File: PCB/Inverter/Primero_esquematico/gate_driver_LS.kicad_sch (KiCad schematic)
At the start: 46 parts

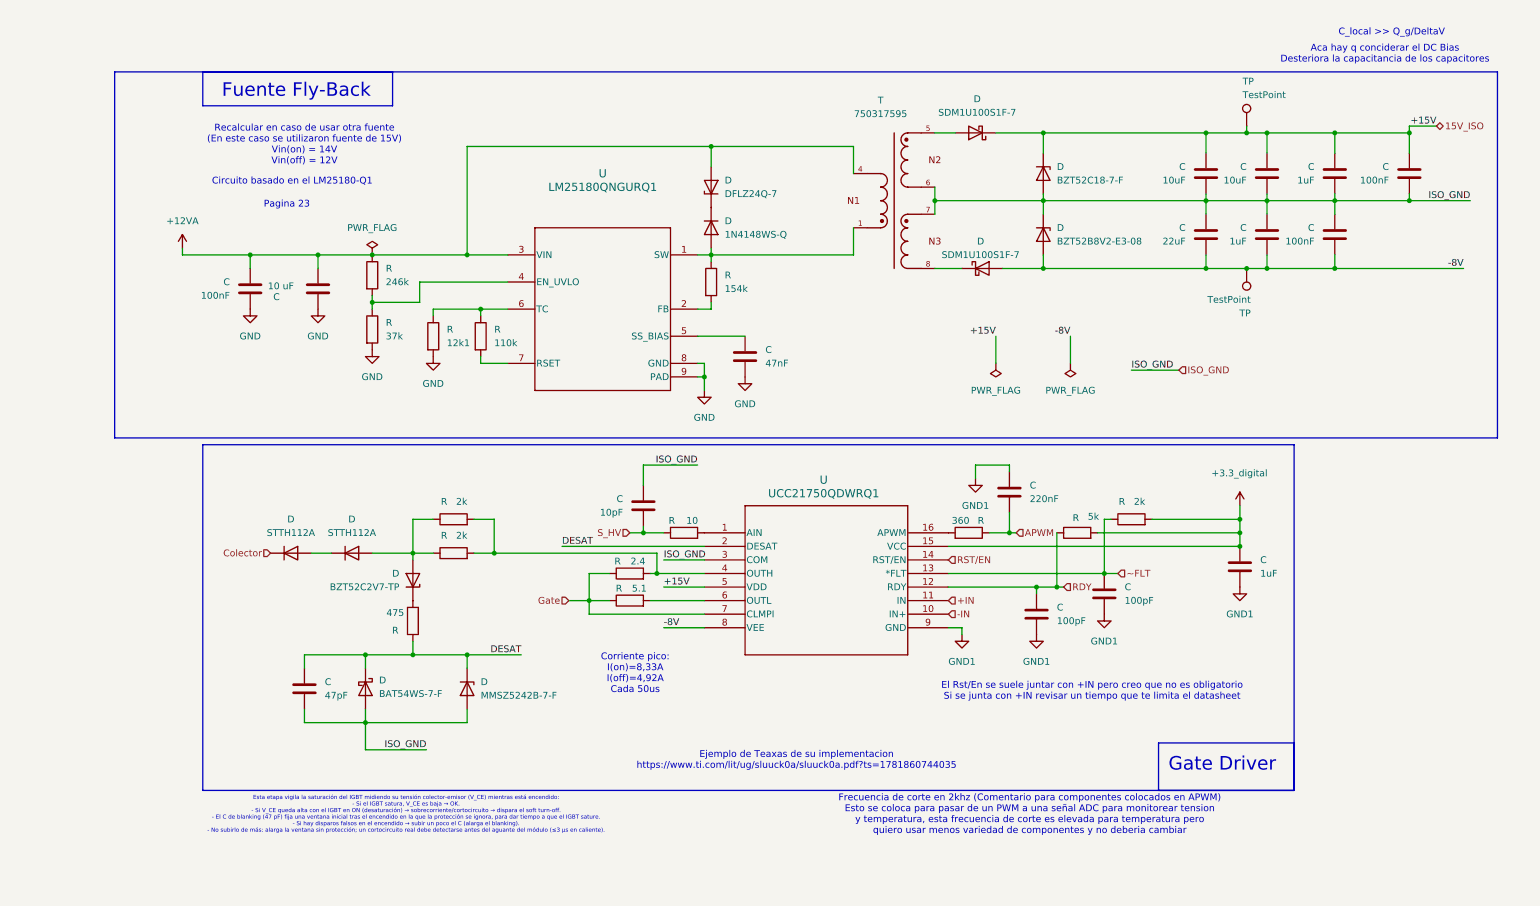
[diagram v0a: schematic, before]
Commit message: Algunos cambios
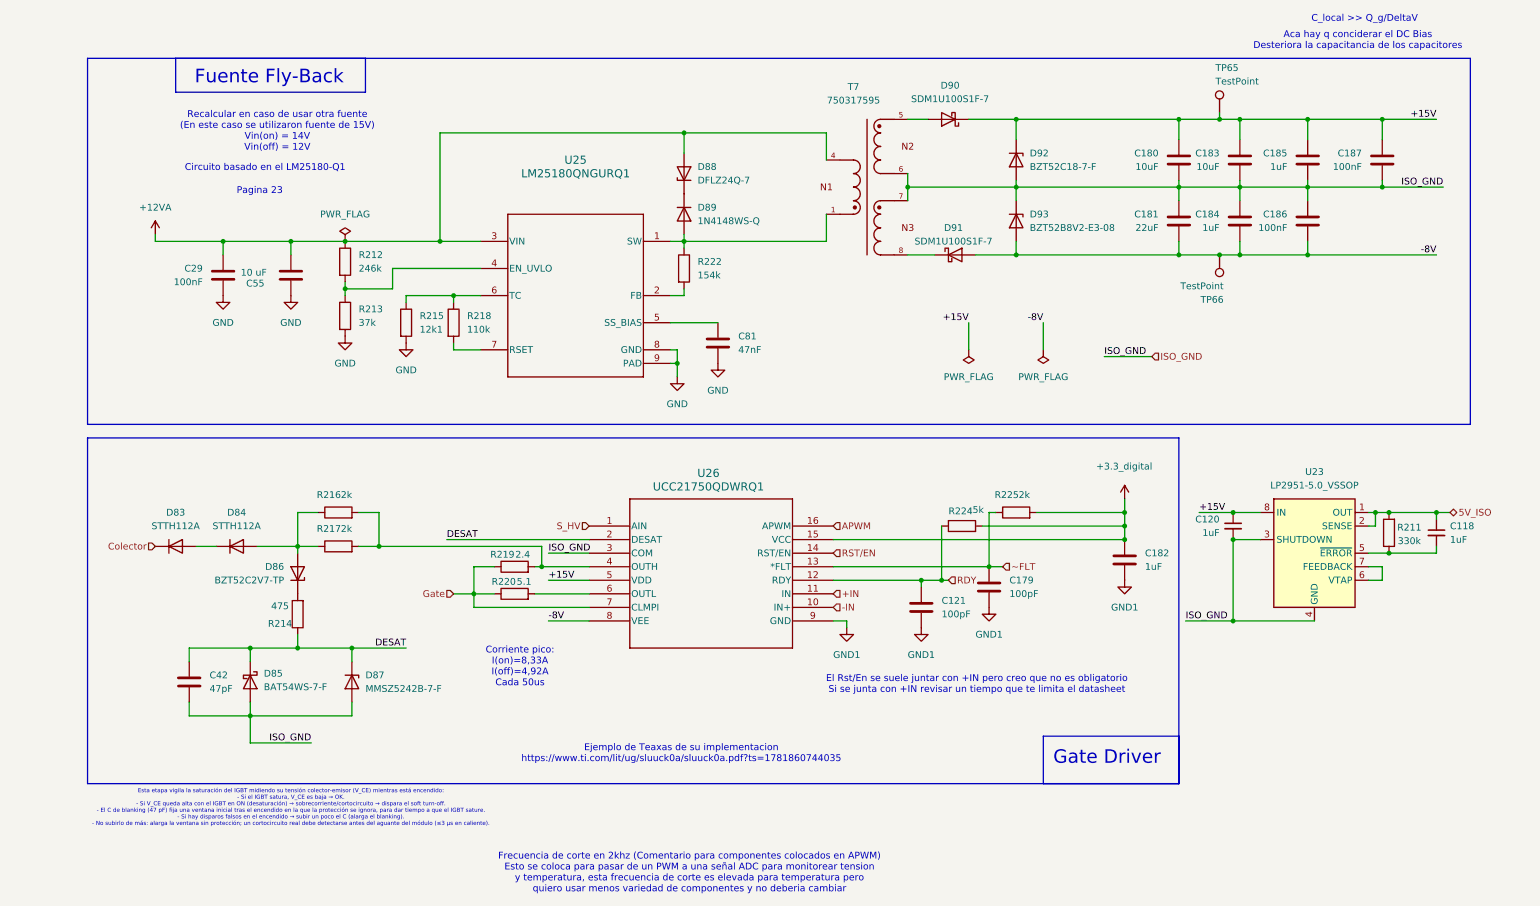
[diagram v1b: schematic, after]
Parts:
- removed C: 10 uF, Capacitor_SMD:C_1206_3216Metric, symbol Device:C
- removed C: 220nF, Capacitor_SMD:C_0402_1005Metric, symbol Device:C
- removed C: 10pF, Capacitor_SMD:C_0402_1005Metric, symbol Device:C
- removed C (x2): 1uF, Capacitor_SMD:C_0805_2012Metric, symbol Device:C
- removed C (x3): 100nF, Capacitor_SMD:C_0402_1005Metric, symbol Device:C
- removed C: 1uF, Capacitor_SMD:C_0603_1608Metric, symbol Device:C
- removed C: 47nF, Capacitor_SMD:C_0402_1005Metric_Pad0.74x0.62mm_HandSolder, symbol Device:C
- removed C: 47pF, Capacitor_SMD:C_0603_1608Metric_Pad1.08x0.95mm_HandSolder, symbol Device:C
- removed C (x2): 10uF, Capacitor_SMD:C_1210_3225Metric, symbol Device:C
- removed C: 22uF, Capacitor_SMD:C_1210_3225Metric, symbol Device:C
- removed C (x2): 100pF, Capacitor_SMD:C_0402_1005Metric, symbol Device:C
- removed D: BZT52C18-7-F, Diode_SMD:D_SOD-123, symbol Device:D_Zener
- removed D (x2): SDM1U100S1F-7, Diode_SMD:D_SOD-123F, symbol Device:D_Schottky
- removed D: MMSZ5242B-7-F, Diode_SMD:D_SOD-123, symbol Device:D_Zener
- removed D: BAT54WS-7-F, Diode_SMD:D_SOD-323_HandSoldering, symbol Device:D_Schottky
- removed D: DFLZ24Q-7, Diode_SMD:D_PowerDI-123, symbol Device:D_Zener
- removed D: 1N4148WS-Q, Diode_SMD:D_SOD-323F, symbol Device:D
- removed D (x2): STTH112A, Diode_SMD:D_SOD-323F, symbol Device:D
- removed D: BZT52B8V2-E3-08, Diode_SMD:D_SOD-123, symbol Device:D_Zener
- removed D: BZT52C2V7-TP, Diode_SMD:D_SOD-123, symbol Device:D_Zener
- removed R: 37k, Resistor_SMD:R_0402_1005Metric, symbol Device:R
- removed R: 5.1, Resistor_SMD:R_1206_3216Metric, symbol Device:R
- removed R: 110k, Resistor_SMD:R_0402_1005Metric, symbol Device:R
- removed R: 10, Resistor_SMD:R_0402_1005Metric, symbol Device:R
- removed R (x2): 2k, Resistor_SMD:R_0805_2012Metric, symbol Device:R
- removed R: 2.4, Resistor_SMD:R_1206_3216Metric, symbol Device:R
- removed R: 246k, Resistor_SMD:R_0402_1005Metric, symbol Device:R
- removed R: 360, Resistor_SMD:R_0402_1005Metric, symbol Device:R
- removed R: 154k, Resistor_SMD:R_0402_1005Metric_Pad0.72x0.64mm_HandSolder, symbol Device:R
- removed R: 475, Resistor_SMD:R_0805_2012Metric, symbol Device:R
- removed R: 12k1, Resistor_SMD:R_0402_1005Metric, symbol Device:R
- removed R: 5k, Resistor_SMD:R_0402_1005Metric, symbol Device:R
- removed R: 2k, Resistor_SMD:R_0402_1005Metric, symbol Device:R
- removed T: 750317595, Snapeda:WE-FLYTI_EP7_4436, symbol Snapeda:750317595
- removed TP (x2): TestPoint, TestPoint:TestPoint_Pad_D1.0mm, symbol Connector:TestPoint
- removed U: UCC21750QDWRQ1, Snapeda:SOIC16_DW_TEX-L, symbol Snapeda:UCC21750QDWRQ1
- removed U: LM25180QNGURQ1, Snapeda:NGU0008C, symbol Snapeda:LM25180QNGURQ1
- added C118, C120: 1uF, Capacitor_SMD:C_0603_1608Metric, symbol Device:C_Small
- added C121, C179: 100pF, Capacitor_SMD:C_0402_1005Metric, symbol Device:C
- added C180, C183: 10uF, Capacitor_SMD:C_1210_3225Metric, symbol Device:C
- added C181: 22uF, Capacitor_SMD:C_1210_3225Metric, symbol Device:C
- added C182: 1uF, Capacitor_SMD:C_0603_1608Metric, symbol Device:C
- added C184, C185: 1uF, Capacitor_SMD:C_0805_2012Metric, symbol Device:C
- added C186, C187, C29: 100nF, Capacitor_SMD:C_0402_1005Metric, symbol Device:C
- added C42: 47pF, Capacitor_SMD:C_0603_1608Metric_Pad1.08x0.95mm_HandSolder, symbol Device:C
- added C55: 10 uF, Capacitor_SMD:C_1206_3216Metric, symbol Device:C
- added C81: 47nF, Capacitor_SMD:C_0402_1005Metric_Pad0.74x0.62mm_HandSolder, symbol Device:C
- added D83, D84: STTH112A, Diode_SMD:D_SOD-323F, symbol Device:D
- added D85: BAT54WS-7-F, Diode_SMD:D_SOD-323_HandSoldering, symbol Device:D_Schottky
- added D86: BZT52C2V7-TP, Diode_SMD:D_SOD-123, symbol Device:D_Zener
- added D87: MMSZ5242B-7-F, Diode_SMD:D_SOD-123, symbol Device:D_Zener
- added D88: DFLZ24Q-7, Diode_SMD:D_PowerDI-123, symbol Device:D_Zener
- added D89: 1N4148WS-Q, Diode_SMD:D_SOD-323F, symbol Device:D
- added D90, D91: SDM1U100S1F-7, Diode_SMD:D_SOD-123F, symbol Device:D_Schottky
- added D92: BZT52C18-7-F, Diode_SMD:D_SOD-123, symbol Device:D_Zener
- added D93: BZT52B8V2-E3-08, Diode_SMD:D_SOD-123, symbol Device:D_Zener
- added R211: 330k, Resistor_SMD:R_0402_1005Metric, symbol Device:R
- added R212: 246k, Resistor_SMD:R_0402_1005Metric, symbol Device:R
- added R213: 37k, Resistor_SMD:R_0402_1005Metric, symbol Device:R
- added R214: 475, Resistor_SMD:R_0805_2012Metric, symbol Device:R
- added R215: 12k1, Resistor_SMD:R_0402_1005Metric, symbol Device:R
- added R216, R217: 2k, Resistor_SMD:R_0805_2012Metric, symbol Device:R
- added R218: 110k, Resistor_SMD:R_0402_1005Metric, symbol Device:R
- added R219: 2.4, Resistor_SMD:R_1206_3216Metric, symbol Device:R
- added R220: 5.1, Resistor_SMD:R_1206_3216Metric, symbol Device:R
- added R222: 154k, Resistor_SMD:R_0402_1005Metric_Pad0.72x0.64mm_HandSolder, symbol Device:R
- added R224: 5k, Resistor_SMD:R_0402_1005Metric, symbol Device:R
- added R225: 2k, Resistor_SMD:R_0402_1005Metric, symbol Device:R
- added T7: 750317595, Snapeda:WE-FLYTI_EP7_4436, symbol Snapeda:750317595
- added TP65, TP66: TestPoint, TestPoint:TestPoint_Pad_D1.0mm, symbol Connector:TestPoint
- added U23: LP2951-5.0_VSSOP, Package_SO:VSSOP-8_3x3mm_P0.65mm, symbol Regulator_Linear:LP2951-5.0_VSSOP
- added U25: LM25180QNGURQ1, Snapeda:NGU0008C, symbol Snapeda:LM25180QNGURQ1
- added U26: UCC21750QDWRQ1, Snapeda:SOIC16_DW_TEX-L, symbol Snapeda:UCC21750QDWRQ1
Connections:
- net +12VA: now also C29.2, C55.1, D88.2 (A), R212.1, T7.4, U25.3 (VIN)
- net +3.3_digital: now also C182.2, R224.2, R225.2, U26.15 (VCC)
- net +IN: now also U26.11 (IN)
- net -8V: now also C181.1, C184.1, C186.1, D91.2 (A), D93.2 (A), TP66.1, U26.8 (VEE)
- net -IN: now also U26.10 (IN+)
- net APWM: now also U26.16 (APWM)
- net Colector: now also D83.1 (K)
- net DESAT: now also C42.2, D85.1 (K), D87.1 (K), R214.1, U26.2 (DESAT)
- net GND: now also C29.1, C55.2, C81.1, R213.2, R215.2, U25.8 (GND), U25.9 (PAD)
- net GND1: now also C121.1, C179.1, C182.1, U26.9 (GND)
- net Gate: now also R219.1, R220.1, U26.7 (CLMPI)
- net ISO_GND: now also C120.2, C180.1, C181.2, C183.1, C184.2, C185.1, C186.2, C187.1, C42.1, D85.2 (A), D87.2 (A), D92.2 (A), D93.1 (K), T7.6, T7.7, U23.3 (SHUTDOWN), U23.4 (GND), U26.3 (COM)
- net RDY: now also C121.2, R224.1, U26.12 (RDY)
- net RST/EN: now also U26.14 (RST/EN)
- net S_HV: now also U26.1 (AIN)
- net ~FLT: now also C179.2, R225.1, U26.13 (*FLT)
- new net: D89.2 (A), R222.1, T7.1, U25.1 (SW)
- new net: R222.2, U25.2 (FB)
- new net: R212.2, R213.1, U25.4 (EN_UVLO)
- new net: C81.2, U25.5 (SS_BIAS)
- new net: R215.1, R218.1, U25.6 (TC)
- new net: R218.2, U25.7 (RSET)
- new net: D88.1 (K), D89.1 (K)
- new net: R216.2, R217.2, R219.2, U26.4 (OUTH)
- new net: D84.2 (A), D86.2 (A), R216.1, R217.1
- new net: D83.2 (A), D84.1 (K)
- new net: C118.2, R211.1, U23.5 (~{ERROR})
- new net: D86.1 (K), R214.2
- new net: D90.2 (A), T7.5
- new net: R220.2, U26.6 (OUTL)
- new net: D91.1 (K), T7.8
- new net: U23.6 (VTAP), U23.7 (FEEDBACK)
- new net +15V: C120.1, C180.2, C183.2, C185.2, C187.2, D90.1 (K), D92.1 (K), TP65.1, U23.8 (IN), U26.5 (VDD)
- new net 5V_ISO: C118.1, R211.2, U23.1 (OUT), U23.2 (SENSE)
